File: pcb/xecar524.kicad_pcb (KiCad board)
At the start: 2 copper layers, 63.8 x 88.9 mm, 39 parts, among them J1 JTAG, J2 PROG, J3 Conn_02x02_Odd_Even, U1 MCP1703A-3302_SOT89, U2 Atari_XE_Cartridge_Connector, U3 XC95144XL-TQ100, U4 SST39VF040

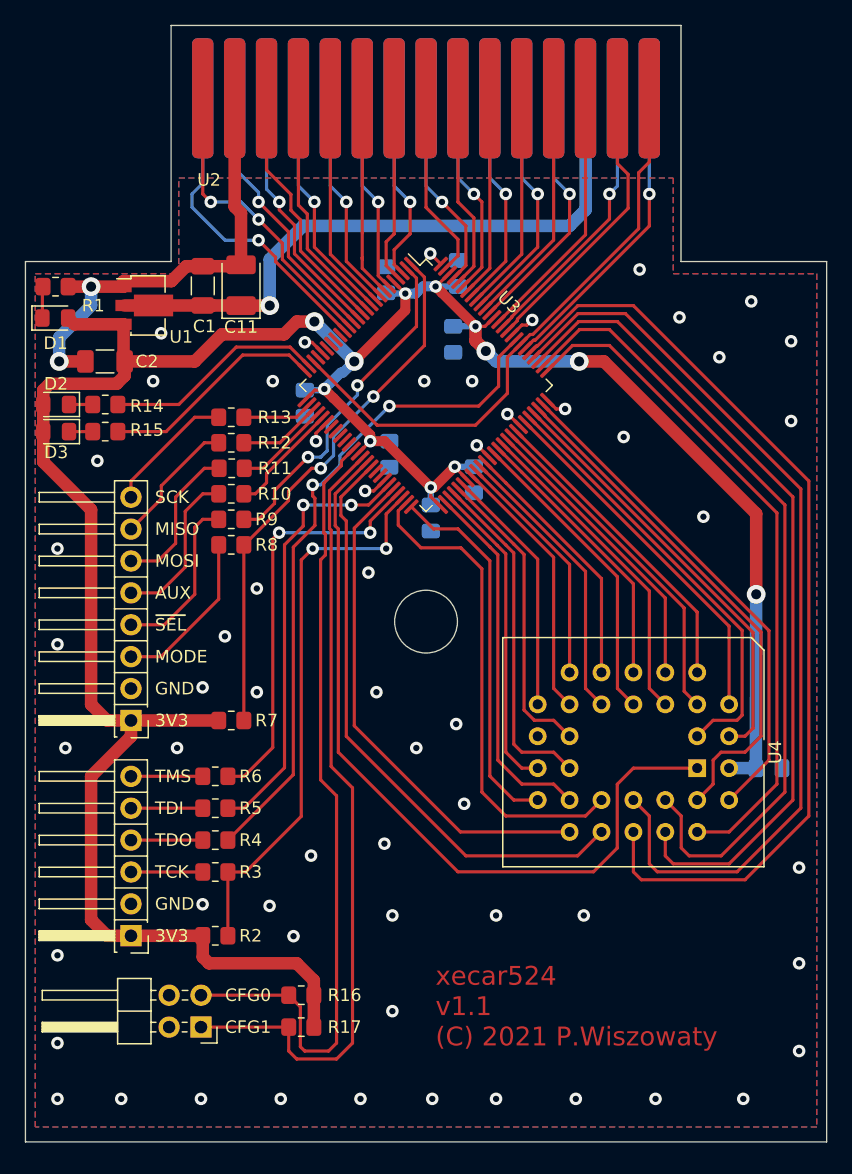
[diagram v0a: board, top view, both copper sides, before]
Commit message: PCB: Resize
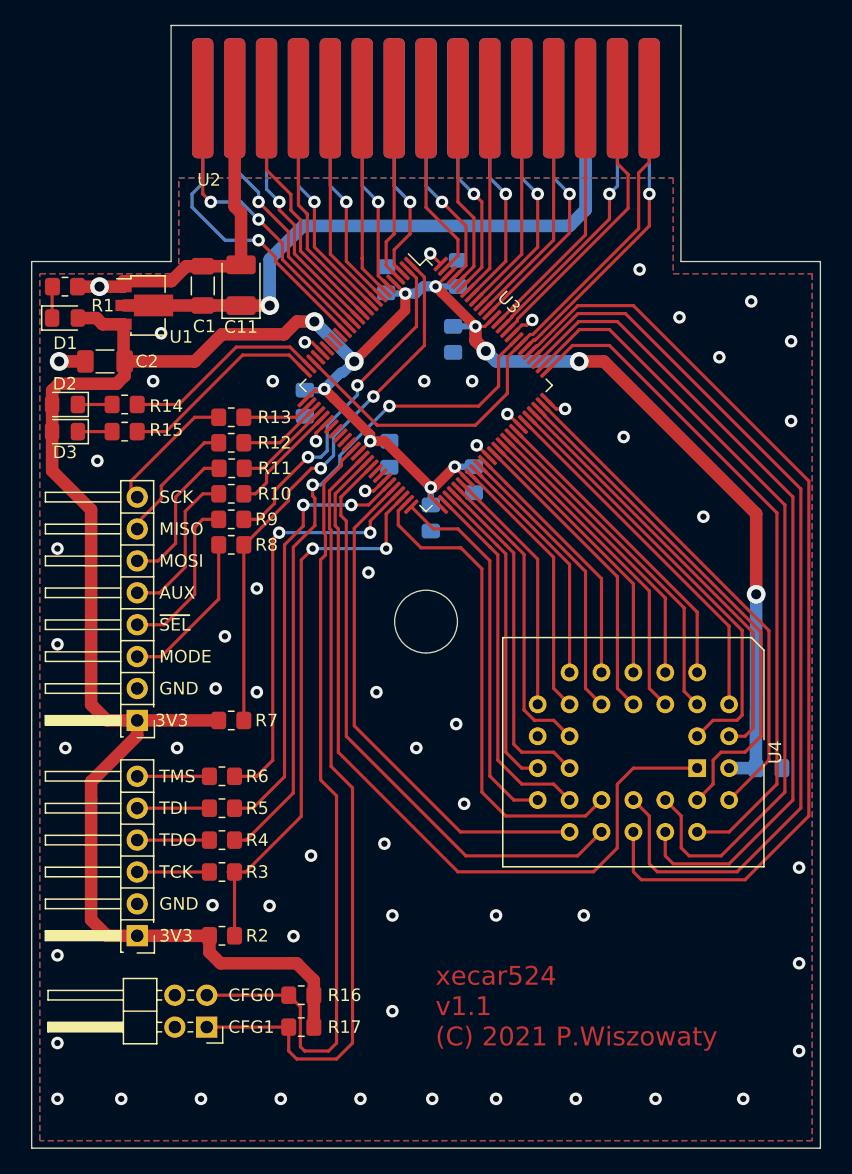
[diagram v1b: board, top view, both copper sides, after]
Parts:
- moved R14 1.54 mm to (126.0, 74.9)
- moved R15 1.54 mm to (126.0, 77.0)
- moved D1 0.78 mm to (121.2, 68.0)
- moved R1 0.75 mm to (121.2, 65.5)
- moved D2 0.70 mm to (121.2, 74.9)
- moved D3 0.70 mm to (121.2, 77.0)
- moved R2 0.53 mm to (133.8, 117.2)
- moved R3 0.53 mm to (133.8, 112.1)
- moved R4 0.53 mm to (133.8, 109.6)
- moved R5 0.53 mm to (133.8, 107.0)
- moved R6 0.53 mm to (133.8, 104.5)
- moved J2 0.50 mm to (127.0, 100.0)
- moved J1 0.50 mm to (127.0, 117.2)
- moved J3 0.46 mm to (132.5, 124.5)
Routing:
- net GND: track 50.8 -> 43.0 mm
- net +3V3: track 221.8 -> 219.0 mm
- net Net-(R15-Pad1): track 17.9 -> 16.4 mm
- net Net-(R14-Pad1): track 17.8 -> 16.2 mm
- net Net-(D3-Pad1): track 1.89 -> 2.72 mm
- net Net-(D2-Pad1): track 1.89 -> 2.72 mm
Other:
- board size 63.8 x 88.9 mm -> 62.8 x 89.4 mm
